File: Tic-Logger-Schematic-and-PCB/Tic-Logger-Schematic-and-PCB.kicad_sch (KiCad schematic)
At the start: 5 parts, among them J1 TFT 1.28 Round Display, J2 MAX30102, J3 MPU6500, U1 ESP32-C3_SUPERMINI_TH

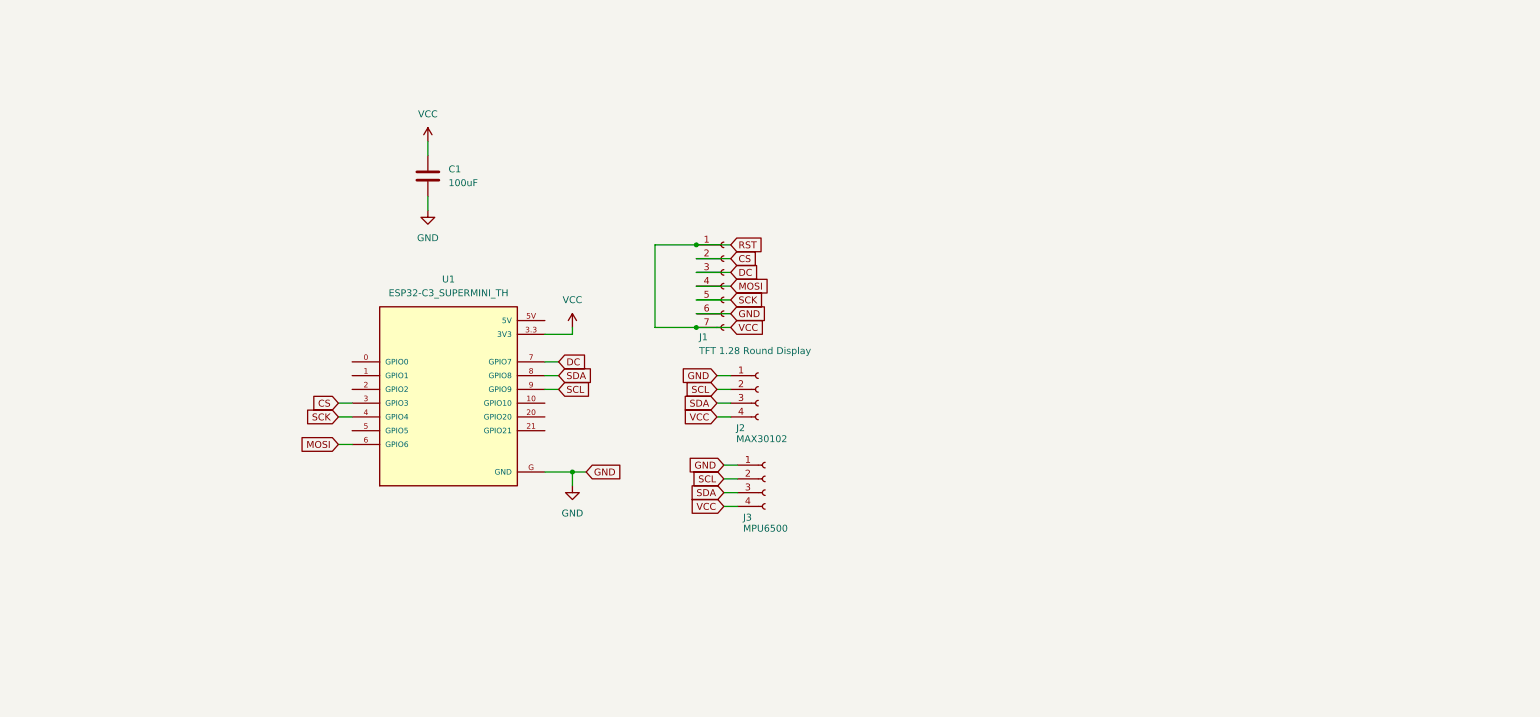
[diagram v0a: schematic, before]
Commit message: update 2
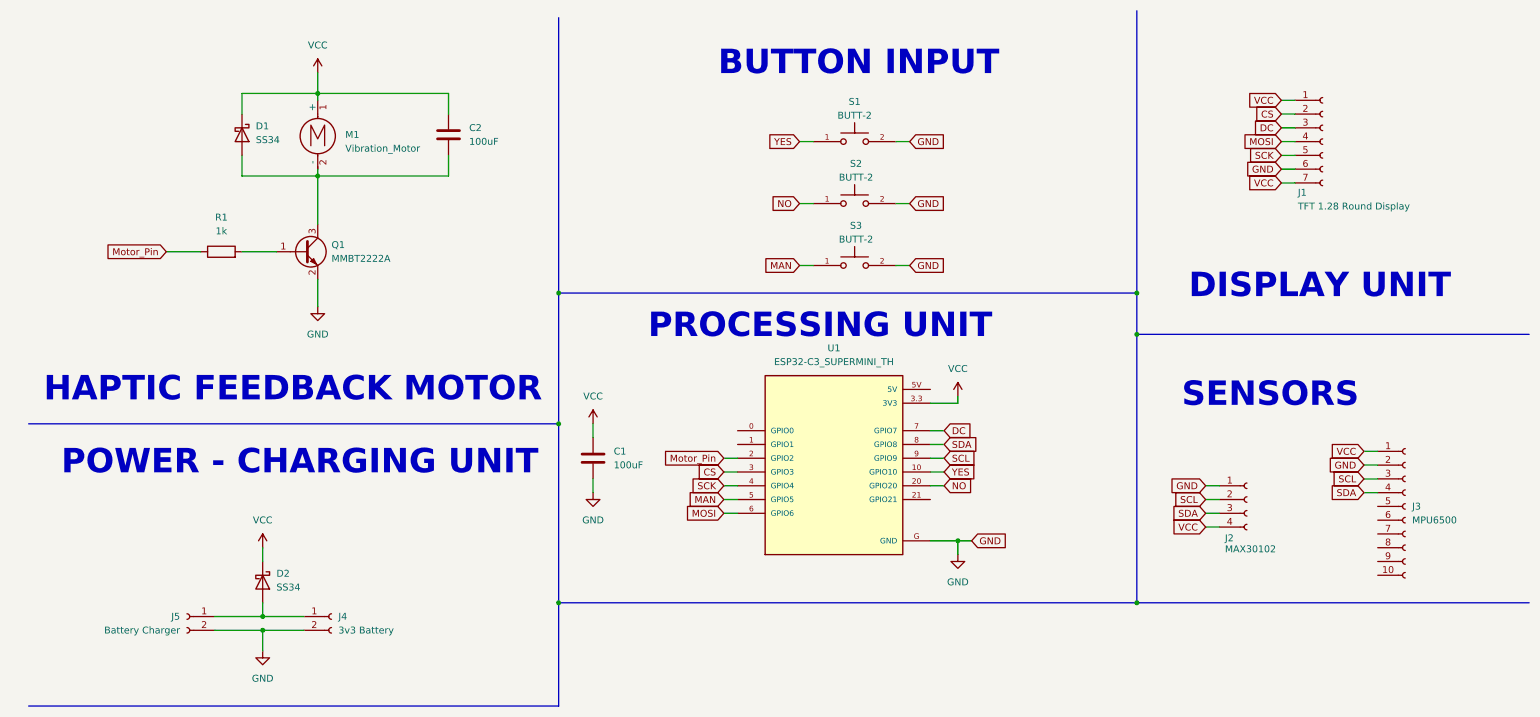
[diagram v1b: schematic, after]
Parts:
- removed J3: MPU6500, Connector_PinSocket_2.54mm:PinSocket_1x04_P2.54mm_Vertical, symbol Connector:Conn_01x04_Socket
- added C2: 100uF, Capacitor_SMD:C_1206_3216Metric, symbol Device:C
- added D1, D2: SS34, Diode_SMD:D_SMA, symbol Diode:SS34
- added J3: MPU6500, Connector_PinSocket_2.54mm:PinSocket_1x10_P2.54mm_Vertical, symbol Connector:Conn_01x10_Socket
- added J4: 3v3 Battery, Connector_JST:JST_PH_B2B-PH-K_1x02_P2.00mm_Vertical, symbol Connector:Conn_01x02_Socket
- added J5: Battery Charger, Connector_JST:JST_PH_B2B-PH-K_1x02_P2.00mm_Vertical, symbol Connector:Conn_01x02_Socket
- added M1: Vibration_Motor, Connector_PinHeader_2.54mm:PinHeader_1x02_P2.54mm_Vertical, symbol Motor:Motor_DC
- added Q1: MMBT2222A, Package_TO_SOT_SMD:SOT-23, symbol Transistor_BJT:MMBT2222A
- added R1: 1k, Resistor_SMD:R_1206_3216Metric, symbol Device:R
- added S1, S2, S3: BUTT-2, KiCad-Additions:SW_BUTT-2, symbol BUTT-2:BUTT-2
- C1: footprint (none) -> Capacitor_SMD:C_1206_3216Metric
- U1: footprint ESP32-C3_SUPERMINI_TH:MODULE_ESP32-C3_SUPERMINI_TH -> KiCad-Additions:MODULE_ESP32-C3_SUPERMINI_TH
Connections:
- net GND: now also J3.2 (Pin_2), J4.2 (Pin_2), J5.2 (Pin_2), Q1.2 (E), S1.2, S2.2, S3.2
- net SCL: now also J3.3 (Pin_3)
- net SDA: now also J3.4 (Pin_4)
- net VCC: now also C2.1, D1.1 (K), D2.1 (K), J3.1 (Pin_1), M1.1 (+)
- net YES: now reaches U1.10 (GPIO10)
- net YES: now also S1.1
- net Motor_Pin: now reaches U1.2 (GPIO2)
- net Motor_Pin: now also R1.1
- net NO: now reaches U1.20 (GPIO20)
- net NO: now also S2.1
- net MAN: now reaches U1.5 (GPIO5)
- net MAN: now also S3.1
- new net: Q1.1 (B), R1.2
- new net: C2.2, D1.2 (A), M1.2 (-), Q1.3 (C)
- new net: D2.2 (A), J4.1 (Pin_1), J5.1 (Pin_1)
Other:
- note added: "BUTTON INPUT"
- note added: "DISPLAY UNIT"
- note added: "HAPTIC FEEDBACK MOTOR"
- note added: "POWER - CHARGING UNIT"
- note added: "PROCESSING UNIT"
- note added: "SENSORS"
- moved on the sheet: C1, J1, J2, U1
